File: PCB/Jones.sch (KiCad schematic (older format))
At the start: 254 parts, among them J1 USB_C_Receptacle_USB2.0, J2 Conn_01x03, J3 Conn_01x02, J5 Conn_02x03_Odd_Even, U1 ATmega32U4-MU, U2 24LC64, Y1 16MHz

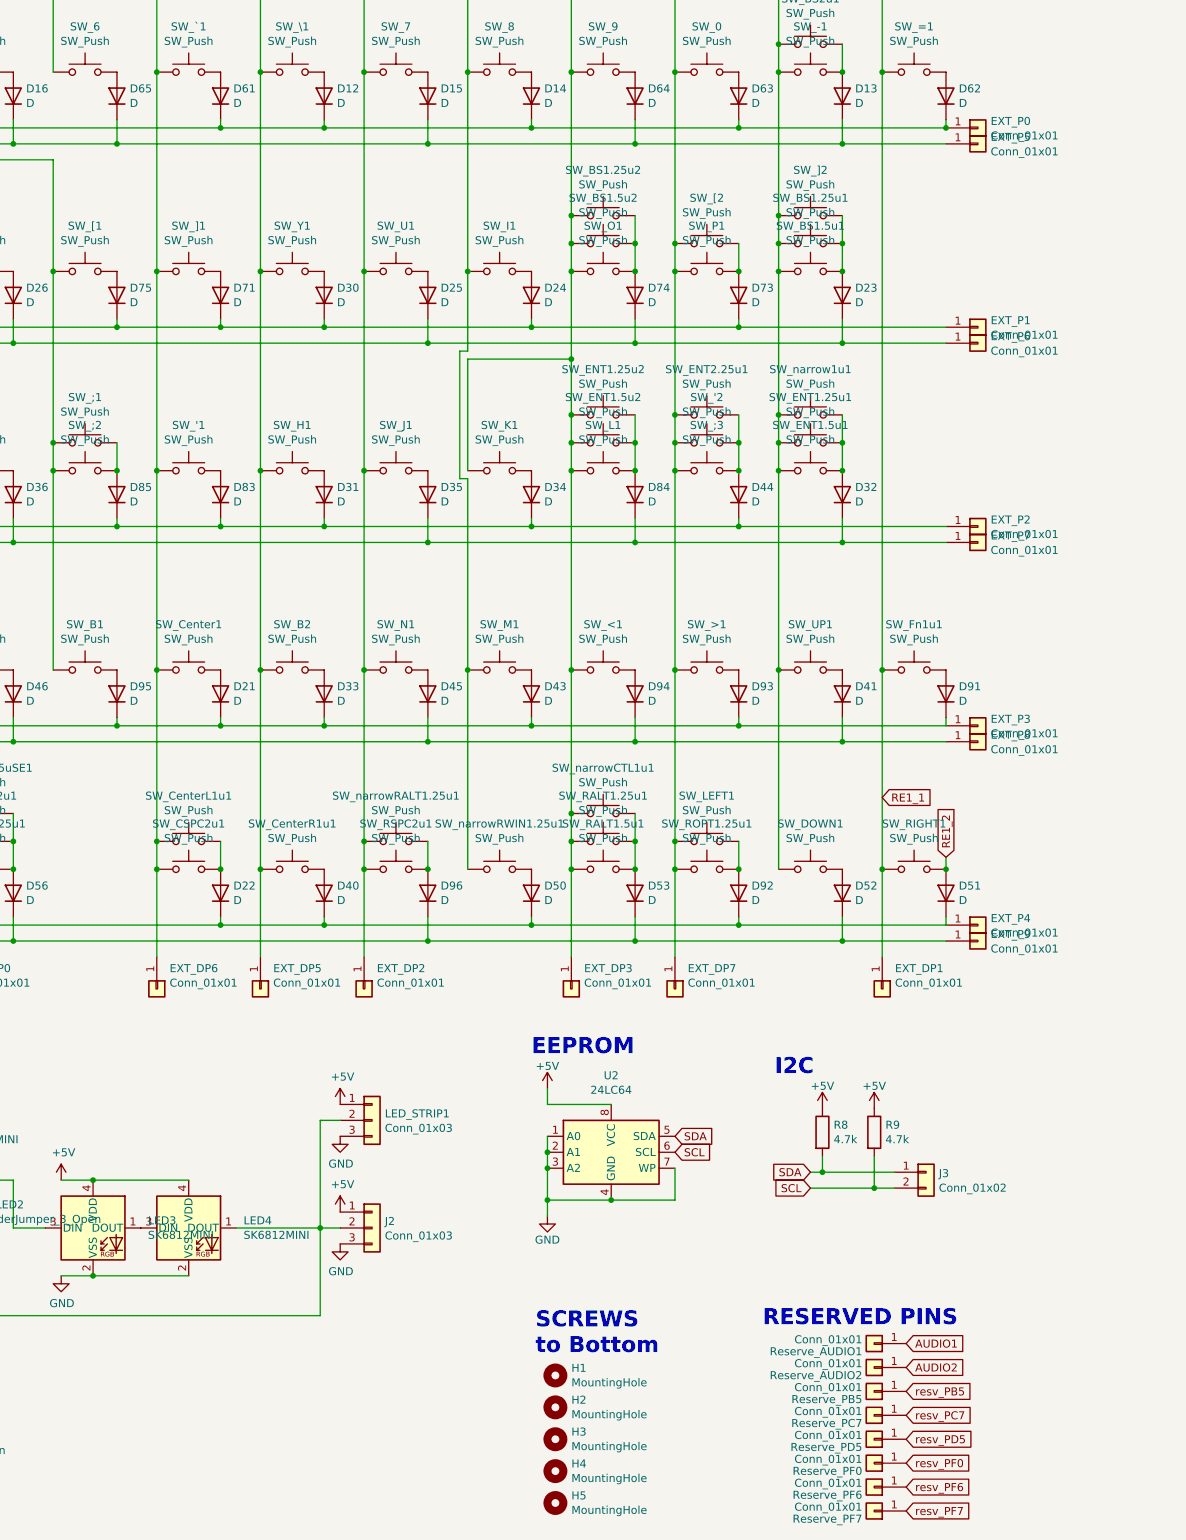
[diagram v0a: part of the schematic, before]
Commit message: WIP：追加：テストピンを何らかの規格のピンヘッダに #18
テストピンまだ

左手側のみ変更
シルクまだ
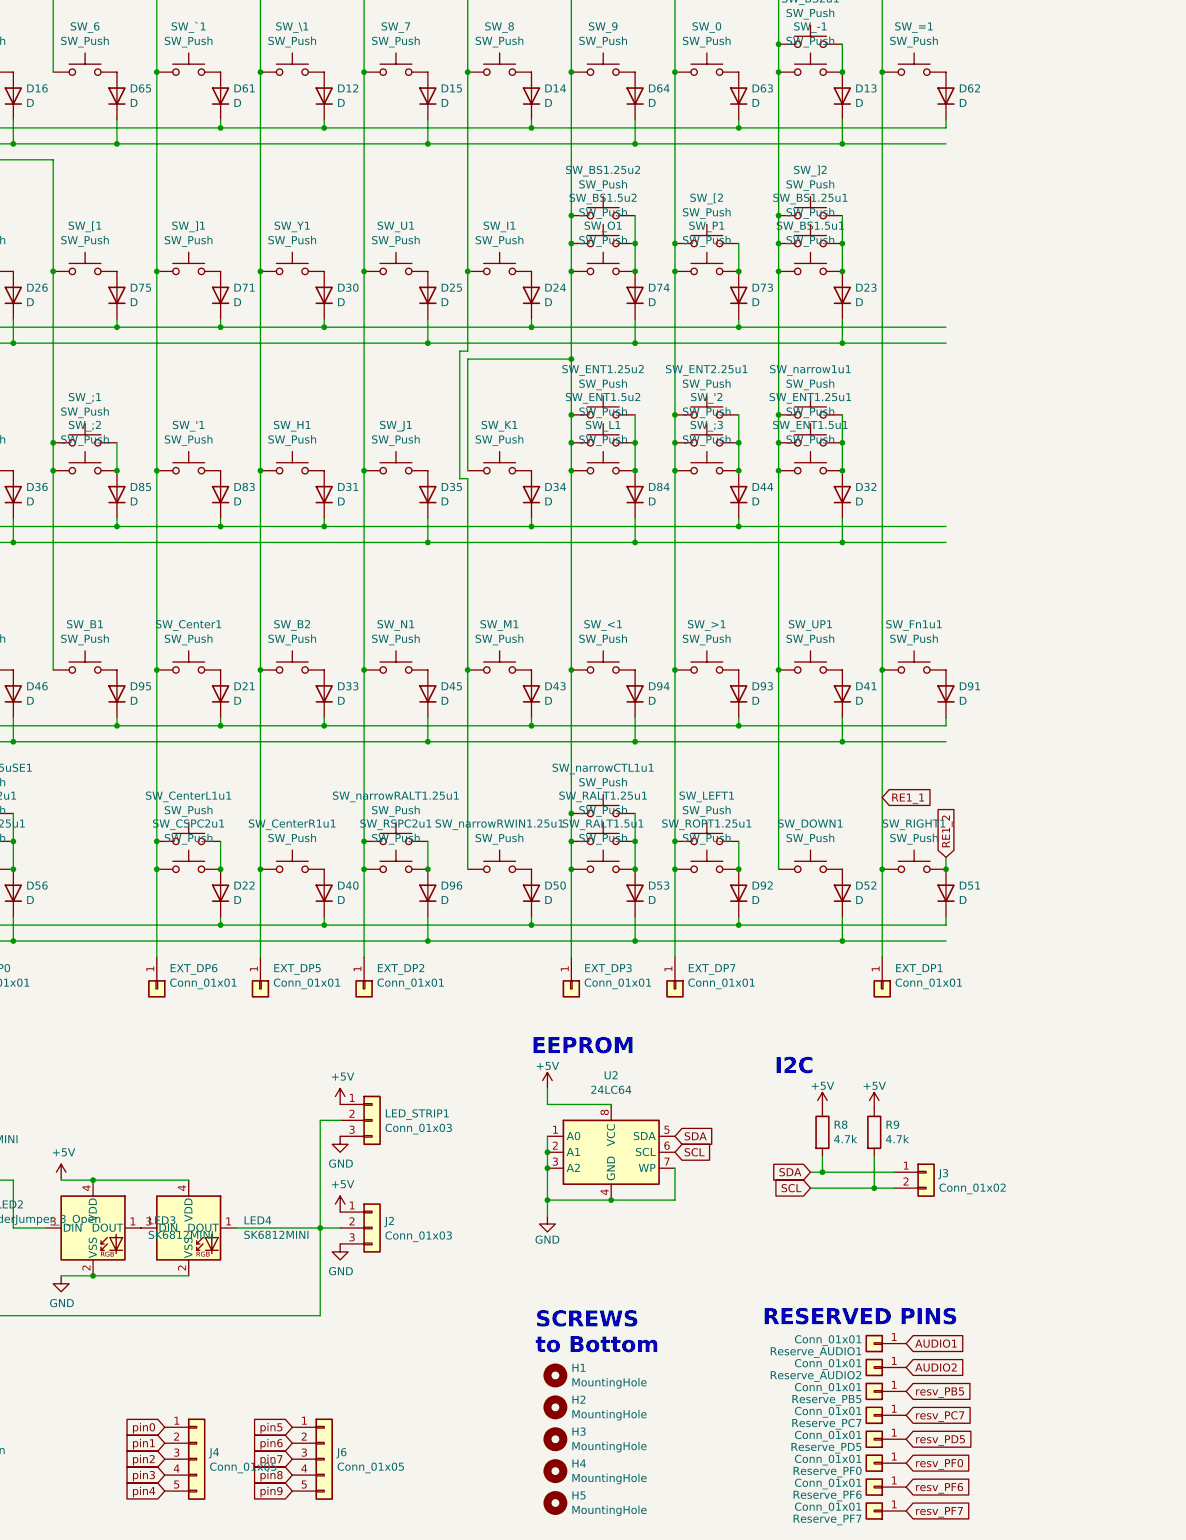
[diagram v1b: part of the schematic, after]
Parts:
- removed EXT_P0, EXT_P1, EXT_P2, EXT_P3, EXT_P4, EXT_P5, EXT_P6, EXT_P7, EXT_P8, EXT_P9: Conn_01x01, TestPoint:TestPoint_THTPad_D1.5mm_Drill0.7mm, symbol Connector_Generic:Conn_01x01
- added J4, J6: Conn_01x05, Connector_PinHeader_2.54mm:PinHeader_1x05_P2.54mm_Vertical, symbol Connector_Generic:Conn_01x05
- SW_LSPC1.25uSE1: footprint MX_Alps_Hybrid:MXOnly-1.25U-Hotswap-guide -> MX_Alps_Hybrid:MXOnly-1.25U-NoLED
- SW_LWIN1.25uSE1: footprint MX_Alps_Hybrid:MXOnly-1.25U-Hotswap-guide-Rotate -> MX_Alps_Hybrid:MXOnly-1.25U-NoLED
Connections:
- net MISO: now also J4.1 (Pin_1)
- net MOSI: now also J4.2 (Pin_2)
- net SCK: now also J6.2 (Pin_2)
- net pin2: now also J4.3 (Pin_3)
- net pin3: now also J4.4 (Pin_4)
- net pin4: now also J4.5 (Pin_5)
- net pin5: now also J6.1 (Pin_1)
- net pin7: now also J6.3 (Pin_3)
- net pin8: now also J6.4 (Pin_4)
- net pin9: now also J6.5 (Pin_5)
